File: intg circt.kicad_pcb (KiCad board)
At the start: 4 copper layers, 18.2 x 40.8 mm, 55 parts, among them J1 Conn_01x01_Pin, J2 USB_C_Receptacle_USB2.0_16P, J3 Conn_01x02_Pin, J4 5033981892, J5 Conn_01x02_Pin, J6 Conn_01x01_Pin, U1 ESP32-S3-MINI-1U, U2 MAXM86161EFD_T, U3 BMI270, U4 BQ24074RGT, U6 USBLC6-2P6, U7 MAX17048X+T10, U8 TLV75533PDBV, U9 LMV358IDR

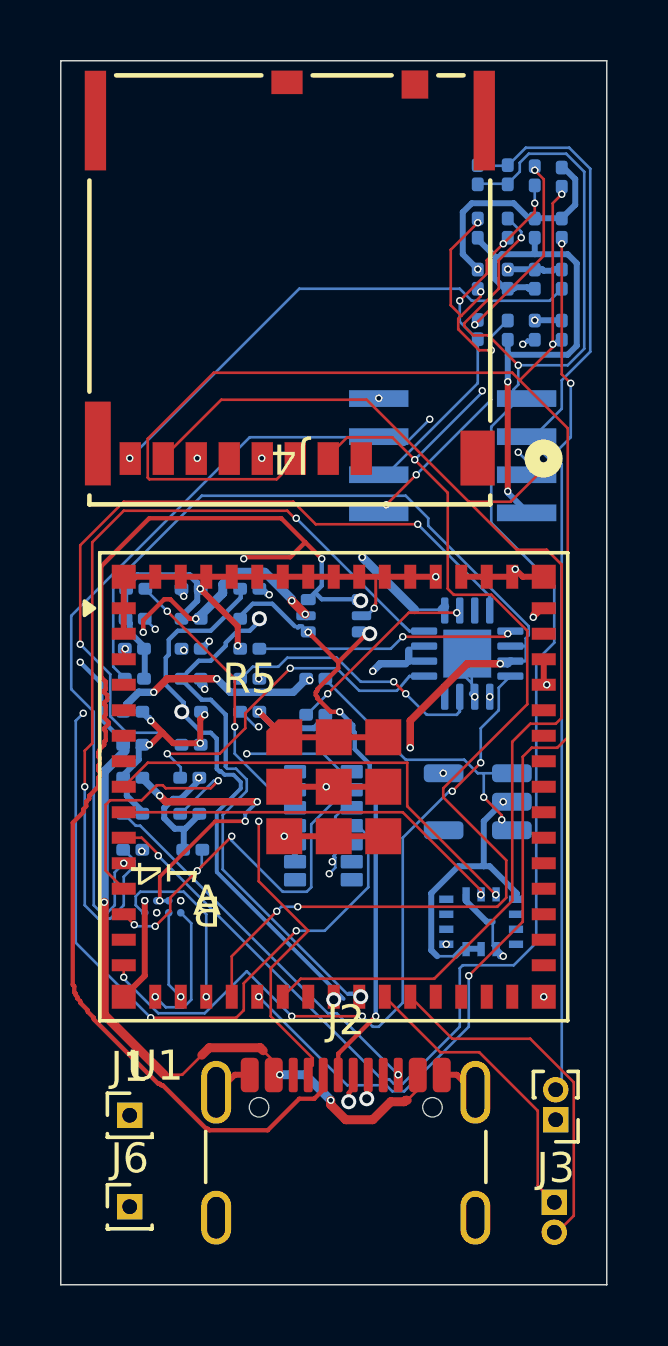
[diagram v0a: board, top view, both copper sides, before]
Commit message: route maxing
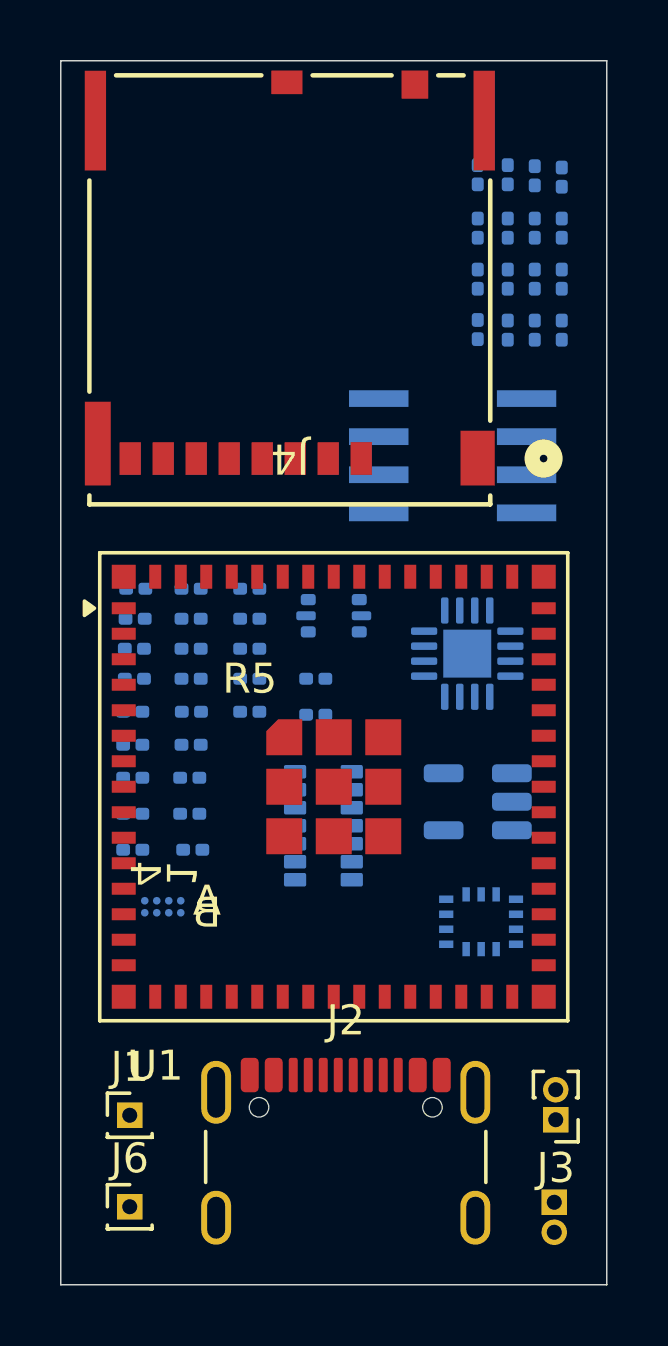
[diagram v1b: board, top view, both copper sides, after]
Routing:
- net GND: track 90.5 -> 0.00 mm, vias 25 -> 0
- net /D-: track 62.6 -> 0.00 mm, vias 5 -> 0
- net /OUT_A: track 61.0 -> 0.00 mm, vias 3 -> 0
- net /J1_CMD: track 60.7 -> 0.00 mm, vias 4 -> 0
- net /J1_DAT0: track 48.9 -> 0.00 mm, vias 3 -> 0
- net /U1_BAT: track 43.3 -> 0.00 mm, vias 6 -> 0
- net /VBUS: track 43.0 -> 0.00 mm, vias 9 -> 0
- net /OUT_B: track 40.9 -> 0.00 mm, vias 5 -> 0
- net /J1_CD: track 39.9 -> 0.00 mm, vias 5 -> 0
- net /D+: track 39.7 -> 0.00 mm, vias 5 -> 0
- net /skin++: track 36.7 -> 0.00 mm
- net Net-(U4-ILIM): track 29.1 -> 0.00 mm, vias 2 -> 0
- net /VLDO: track 27.6 -> 0.00 mm, vias 4 -> 0
- net Net-(U4-ISET): track 24.9 -> 0.00 mm, vias 2 -> 0
- net +3V3: track 24.9 -> 0.00 mm, vias 17 -> 0
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- removed copper zone on In2.Cu, net +3V3
- removed copper zone on In1.Cu, net GND
